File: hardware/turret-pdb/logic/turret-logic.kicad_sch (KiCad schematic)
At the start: 14 parts, among them J12 Stack link, J5 ESC left, J6 ESC right, J7 TTLinker, J8 TFmini Plus, J9 Light gate, U1 Freenove ESP32-S3 WROOM, U2 Adafruit 757

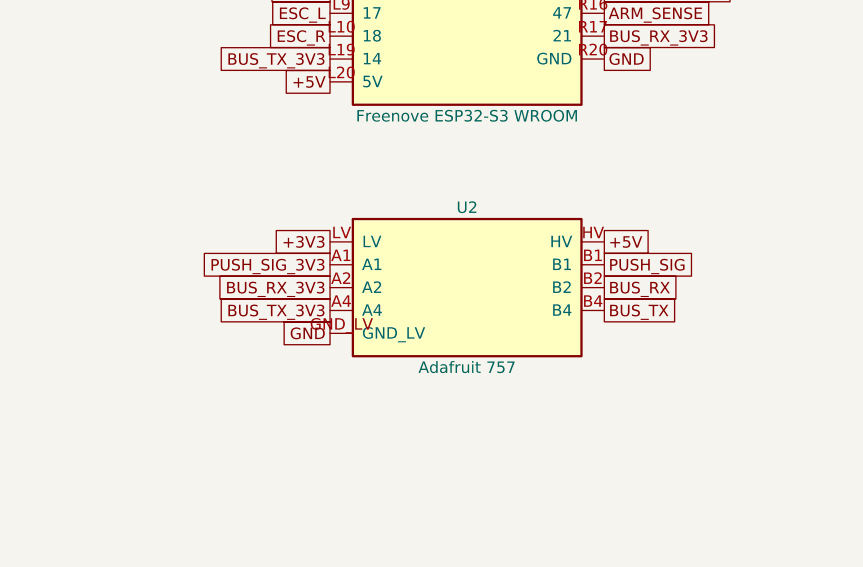
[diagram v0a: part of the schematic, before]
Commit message: Route the logic board
Co-Authored-By: Claude Opus 5.5 <noreply@anthropic.com>
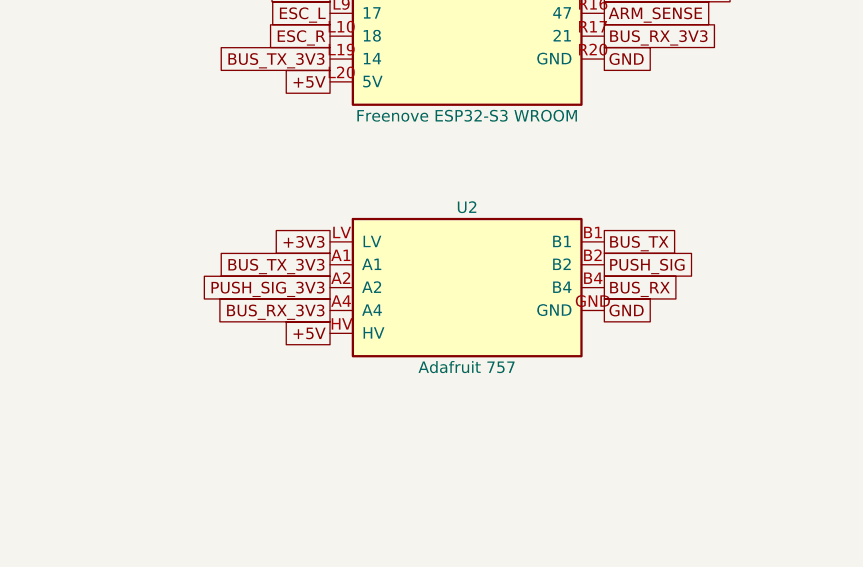
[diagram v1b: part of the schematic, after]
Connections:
- net BUS_RX: now also U2.B4; no longer U2.B2
- net BUS_RX_3V3: now also U2.A4; no longer U2.A2
- net BUS_TX: now also U2.B1; no longer U2.B4
- net BUS_TX_3V3: now also U2.A1; no longer U2.A4
- net GND: now also U2.GND; no longer U2.GND_LV
- net PUSH_SIG: now also U2.B2; no longer U2.B1
- net PUSH_SIG_3V3: now also U2.A2; no longer U2.A1
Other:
- moved on the sheet: U2
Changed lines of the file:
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@@
 		(pin "A4"
 		)
-		(pin "GND_LV"
-		)
 		(pin "HV"
 		)
@@
 		)
 		(pin "B4"
+		)
+		(pin "GND"
 		)
 		(instances
@@
 		)
 	)
+	(global_label "BUS_TX_3V3"
+		(shape passive)
+		(at 99.06 68.58 180)
+		(fields_autoplaced yes)
+		(effects
+			(font
+				(size 1.27 1.27)
+			)
+			(justify right)
+		)
+		(property "Intersheetrefs" "${INTERSHEET_REFS}"
+			(at 99.06 68.58 0)
+			(effects
+				(font
+					(size 1.27 1.27)
+				)
+				(hide yes)
+			)
+		)
+	)
 	(global_label "PUSH_SIG_3V3"
 		(shape passive)
-		(at 99.06 68.58 180)
+		(at 99.06 71.12 180)
 		(fields_autoplaced yes)
 		(effects
@@
 		)
 		(property "Intersheetrefs" "${INTERSHEET_REFS}"
-			(at 99.06 68.58 0)
+			(at 99.06 71.12 0)
 			(effects
 				(font
@@
 	(global_label "BUS_RX_3V3"
 		(shape passive)
-		(at 99.06 71.12 180)
+		(at 99.06 73.66 180)
 		(fields_autoplaced yes)
 		(effects
@@
 		)
 		(property "Intersheetrefs" "${INTERSHEET_REFS}"
-			(at 99.06 71.12 0)
-			(effects
-				(font
-					(size 1.27 1.27)
-				)
-				(hide yes)
-			)
-		)
-	)
-	(global_label "BUS_TX_3V3"
-		(shape passive)
-		(at 99.06 73.66 180)
+			(at 99.06 73.66 0)
+			(effects
+				(font
+					(size 1.27 1.27)
+				)
+				(hide yes)
+			)
+		)
+	)
+	(global_label "+5V"
+		(shape passive)
+		(at 99.06 76.2 180)
 		(fields_autoplaced yes)
 		(effects
@@
 		)
 		(property "Intersheetrefs" "${INTERSHEET_REFS}"
-			(at 99.06 73.66 0)
+			(at 99.06 76.2 0)
+			(effects
+				(font
+					(size 1.27 1.27)
+				)
+				(hide yes)
+			)
+		)
+	)
+	(global_label "BUS_TX"
+		(shape passive)
+		(at 129.54 66.04 0)
+		(fields_autoplaced yes)
+		(effects
+			(font
+				(size 1.27 1.27)
+			)
+			(justify left)
+		)
+		(property "Intersheetrefs" "${INTERSHEET_REFS}"
+			(at 129.54 66.04 0)
+			(effects
+				(font
+					(size 1.27 1.27)
+				)
+				(hide yes)
+			)
+		)
+	)
+	(global_label "PUSH_SIG"
+		(shape passive)
+		(at 129.54 68.58 0)
+		(fields_autoplaced yes)
+		(effects
+			(font
+				(size 1.27 1.27)
+			)
+			(justify left)
+		)
+		(property "Intersheetrefs" "${INTERSHEET_REFS}"
+			(at 129.54 68.58 0)
+			(effects
+				(font
+					(size 1.27 1.27)
+				)
+				(hide yes)
+			)
+		)
+	)
+	(global_label "BUS_RX"
+		(shape passive)
+		(at 129.54 71.12 0)
+		(fields_autoplaced yes)
+		(effects
+			(font
+				(size 1.27 1.27)
+			)
+			(justify left)
+		)
+		(property "Intersheetrefs" "${INTERSHEET_REFS}"
+			(at 129.54 71.12 0)
 			(effects
 				(font
@@
 	(global_label "GND"
 		(shape passive)
-		(at 99.06 76.2 180)
-		(fields_autoplaced yes)
-		(effects
-			(font
-				(size 1.27 1.27)
-			)
-			(justify right)
-		)
-		(property "Intersheetrefs" "${INTERSHEET_REFS}"
-			(at 99.06 76.2 0)
-			(effects
-				(font
-					(size 1.27 1.27)
-				)
-				(hide yes)
-			)
-		)
-	)
-	(global_label "+5V"
-		(shape passive)
-		(at 129.54 66.04 0)
-		(fields_autoplaced yes)
-		(effects
-			(font
-				(size 1.27 1.27)
-			)
-			(justify left)
-		)
-		(property "Intersheetrefs" "${INTERSHEET_REFS}"
-			(at 129.54 66.04 0)
-			(effects
-				(font
-					(size 1.27 1.27)
-				)
-				(hide yes)
-			)
-		)
-	)
-	(global_label "PUSH_SIG"
-		(shape passive)
-		(at 129.54 68.58 0)
-		(fields_autoplaced yes)
-		(effects
-			(font
-				(size 1.27 1.27)
-			)
-			(justify left)
-		)
-		(property "Intersheetrefs" "${INTERSHEET_REFS}"
-			(at 129.54 68.58 0)
-			(effects
-				(font
-					(size 1.27 1.27)
-				)
-				(hide yes)
-			)
-		)
-	)
-	(global_label "BUS_RX"
-		(shape passive)
-		(at 129.54 71.12 0)
-		(fields_autoplaced yes)
-		(effects
-			(font
-				(size 1.27 1.27)
-			)
-			(justify left)
-		)
-		(property "Intersheetrefs" "${INTERSHEET_REFS}"
-			(at 129.54 71.12 0)
-			(effects
-				(font
-					(size 1.27 1.27)
-				)
-				(hide yes)
-			)
-		)
-	)
-	(global_label "BUS_TX"
-		(shape passive)
 		(at 129.54 73.66 0)
